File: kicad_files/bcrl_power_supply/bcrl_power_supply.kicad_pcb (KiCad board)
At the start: 2 copper layers, 16 parts, among them J1 OSTVN02A150, J2 OSTVN02A150, J3 OSTVN02A150, J4 OSTVN02A150, J5 OSTVN02A150, J6 OSTVN02A150, J7 OSTVN02A150, J8 OSTVN02A150, P1 Conn_01x10, P2 Conn_01x10, P3 Conn_01x10, P4 Conn_01x10

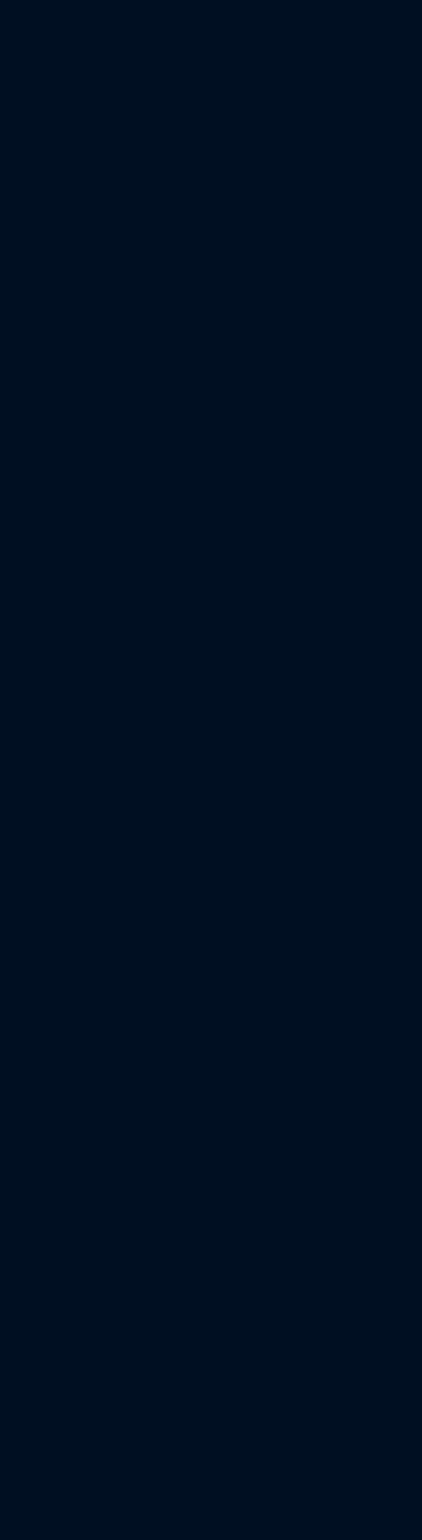
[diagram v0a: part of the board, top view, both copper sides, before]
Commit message: fixed path
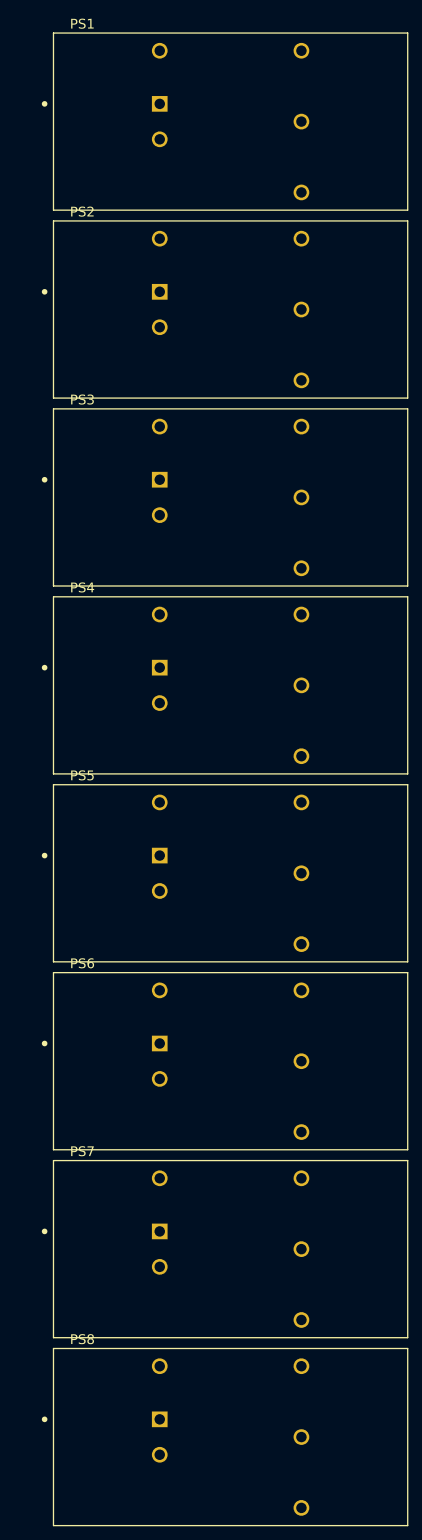
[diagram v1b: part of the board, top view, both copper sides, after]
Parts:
- added PS1: PYBE20-Q48-S9, BCRL_power_supply:CONV_PYBE20-Q48-S9, F.Cu at (193.0, -41.5)
- added PS2: PYBE20-Q48-S9, BCRL_power_supply:CONV_PYBE20-Q48-S9, F.Cu at (193.0, -14.5)
- added PS3: PYBE20-Q48-S9, BCRL_power_supply:CONV_PYBE20-Q48-S9, F.Cu at (193.0, 12.4)
- added PS4: PYBE20-Q48-S9, BCRL_power_supply:CONV_PYBE20-Q48-S9, F.Cu at (193.0, 39.4)
- added PS5: PYBE20-Q48-S5, BCRL_power_supply:CONV_PYBE20-Q48-S5, F.Cu at (193.0, 66.3)
- added PS6: PYBE20-Q48-S5, BCRL_power_supply:CONV_PYBE20-Q48-S5, F.Cu at (193.0, 93.3)
- added PS7: PYBE20-Q48-S5, BCRL_power_supply:CONV_PYBE20-Q48-S5, F.Cu at (193.0, 120.2)
- added PS8: PYBE20-Q48-S5, BCRL_power_supply:CONV_PYBE20-Q48-S5, F.Cu at (193.0, 147.2)
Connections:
- J1 pad 1: 48V -> unconnected-(J1-Pad1)
- J1 pad 2: 48V -> unconnected-(J1-Pad2)
- J2 pad 1: 48V -> unconnected-(J2-Pad1)
- J2 pad 2: 48V -> unconnected-(J2-Pad2)
- J3 pad 1: GND -> unconnected-(J3-Pad1)
- J3 pad 2: GND -> unconnected-(J3-Pad2)
- J4 pad 1: GND -> unconnected-(J4-Pad1)
- J4 pad 2: GND -> unconnected-(J4-Pad2)
